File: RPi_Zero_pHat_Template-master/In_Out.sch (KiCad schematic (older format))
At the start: 34 parts, among them J3 DHT22 Conn, J4 HD38 Conn, J5 120VAC, J6 R_Si, J7 Ventilador, J8 Bomba Agua, J9 Tira LED, Q1 BT136-500, Q2 MMBT2222A, Q3 MMBT2222A, U4 LM35, U5 MOC3011M, U8 TLP3543

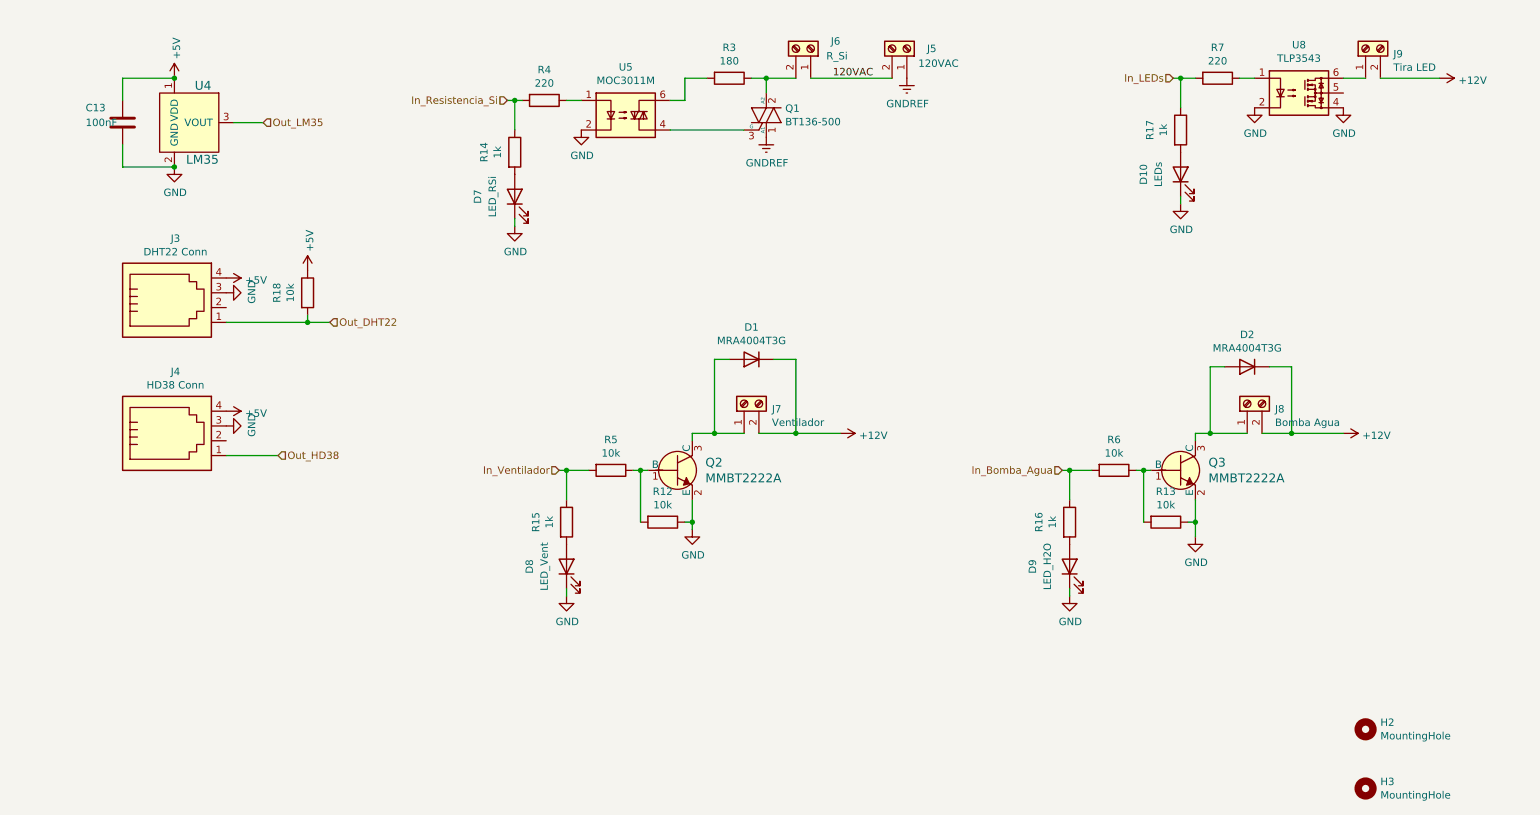
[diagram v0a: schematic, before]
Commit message: Archivos KiCad
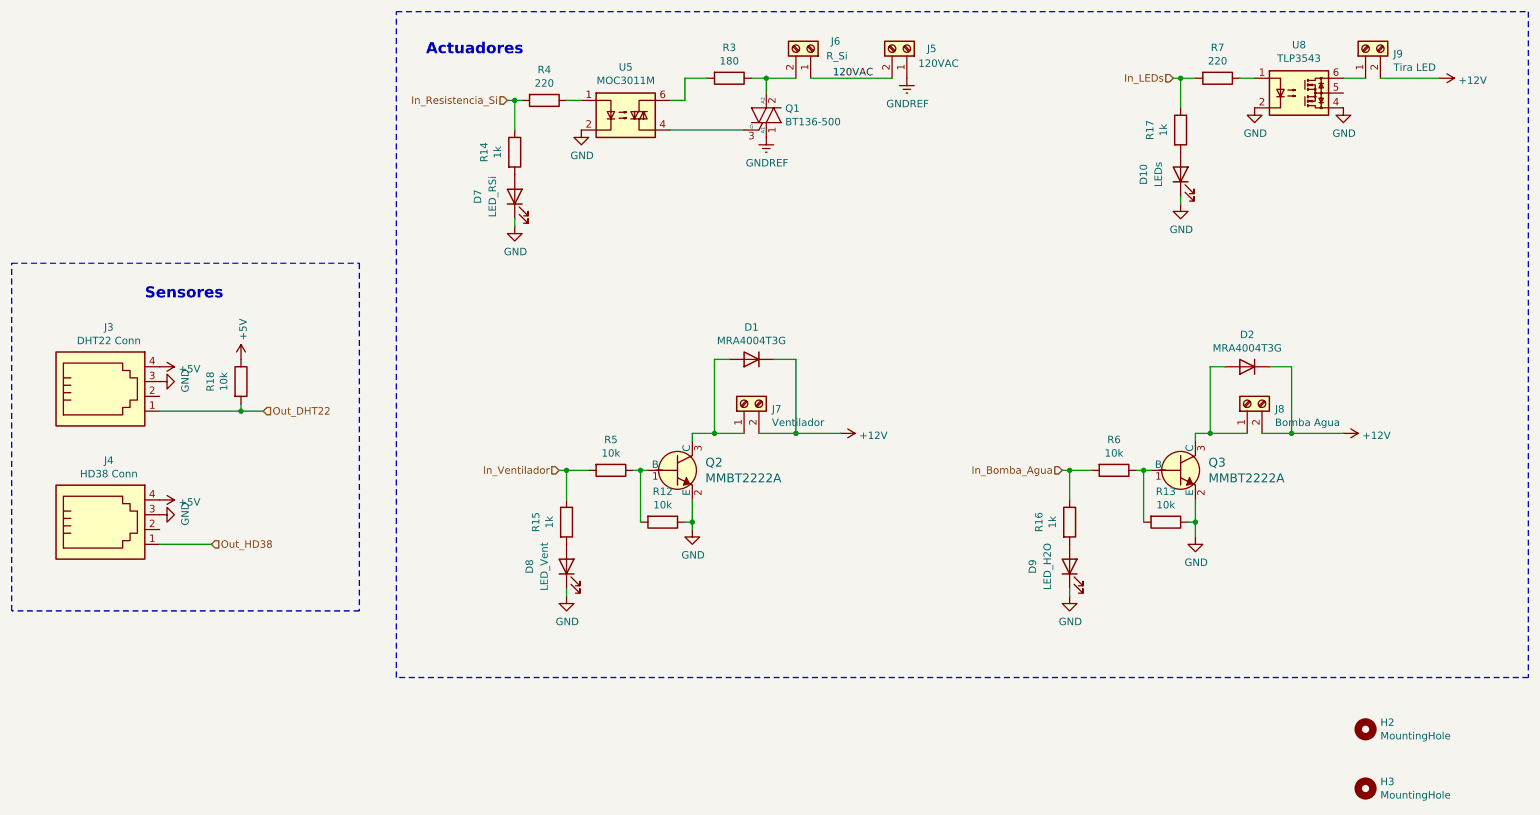
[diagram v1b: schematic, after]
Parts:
- removed C13: 100nF, Capacitor_SMD:C_0805_2012Metric, symbol Device:C
- removed U4: LM35, digikey-footprints:SOIC-8_W3.9mm, symbol dk_Temperature-Sensors-Analog-and-Digital-Output:LM35DT_NOPB
- J3, J4: footprint RJ9-Conn:520249-2 -> RJ9-Conn:RJ9-4P4C
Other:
- note added: "Actuadores"
- note added: "Sensores"
- moved on the sheet: J3, J4, R18
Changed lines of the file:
@@
 $EndDescr
-$Comp
-L dk_Temperature-Sensors-Analog-and-Digital-Output:LM35DT_NOPB U?
-U 1 1 608216FC
-P 1800 1500
-AR Path="/608216FC" Ref="U?"  Part="1"
-AR Path="/6081C49D/608216FC" Ref="U4"  Part="1"
-F 0 "U4" H 2050 1750 60  0000 R CNN
-F 1 "LM35" H 2100 1250 60  0000 R CNN
-F 2 "digikey-footprints:SOIC-8_W3.9mm" H 2000 1700 60  0001 L CNN
-F 3 "http://www.ti.com/general/docs/suppproductinfo.tsp?distId=10&gotoUrl=http%3A%2F%2Fwww.ti.com%2Flit%2Fgpn%2Flm35" H 2000 1800 60  0001 L CNN
-F 4 "LM35DT/NOPB-ND" H 2000 1900 60  0001 L CNN "Digi-Key_PN"
-F 5 "LM35DT/NOPB" H 2000 2000 60  0001 L CNN "MPN"
-F 6 "Sensors, Transducers" H 2000 2100 60  0001 L CNN "Category"
-F 7 "Temperature Sensors - Analog and Digital Output" H 2000 2200 60  0001 L CNN "Family"
-F 8 "http://www.ti.com/general/docs/suppproductinfo.tsp?distId=10&gotoUrl=http%3A%2F%2Fwww.ti.com%2Flit%2Fgpn%2Flm35" H 2000 2300 60  0001 L CNN "DK_Datasheet_Link"
-F 9 "/product-detail/en/texas-instruments/LM35DT-NOPB/LM35DT-NOPB-ND/362706" H 2000 2400 60  0001 L CNN "DK_Detail_Page"
-F 10 "SENSOR ANALOG 0C-100C TO220-3" H 2000 2500 60  0001 L CNN "Description"
-F 11 "Texas Instruments" H 2000 2600 60  0001 L CNN "Manufacturer"
-F 12 "Active" H 2000 2700 60  0001 L CNN "Status"
-	1    1800 1500
-	1    0    0    -1
-$EndComp
-$Comp
-L power:+5V #PWR?
-U 1 1 60821702
-P 1800 1200
-AR Path="/60821702" Ref="#PWR?"  Part="1"
-AR Path="/6081C49D/60821702" Ref="#PWR0130"  Part="1"
-F 0 "#PWR0130" H 1800 1050 50  0001 C CNN
-F 1 "+5V" V 1815 1328 50  0000 L CNN
-F 2 "" H 1800 1200 50  0001 C CNN
-F 3 "" H 1800 1200 50  0001 C CNN
-	1    1800 1200
-	1    0    0    -1
-$EndComp
-$Comp
-L power:GND #PWR?
-U 1 1 60821708
-P 1800 1800
-AR Path="/60821708" Ref="#PWR?"  Part="1"
-AR Path="/6081C49D/60821708" Ref="#PWR0131"  Part="1"
-F 0 "#PWR0131" H 1800 1550 50  0001 C CNN
-F 1 "GND" H 1805 1627 50  0000 C CNN
-F 2 "" H 1800 1800 50  0001 C CNN
-F 3 "" H 1800 1800 50  0001 C CNN
-	1    1800 1800
-	1    0    0    -1
-$EndComp
-Wire Wire Line
-	1450 1350 1450 1200
-Wire Wire Line
-	1450 1200 1800 1200
-Wire Wire Line
-	1450 1650 1450 1800
-Wire Wire Line
-	1450 1800 1800 1800
-Connection ~ 1800 1800
-$Comp
-L Device:C C?
-U 1 1 60821713
-P 1450 1500
-AR Path="/60821713" Ref="C?"  Part="1"
-AR Path="/6081C49D/60821713" Ref="C13"  Part="1"
-F 0 "C13" H 1200 1600 50  0000 L CNN
-F 1 "100nF" H 1200 1500 50  0000 L CNN
-F 2 "Capacitor_SMD:C_0805_2012Metric" H 1488 1350 50  0001 C CNN
-F 3 "~" H 1450 1500 50  0001 C CNN
-	1    1450 1500
-	1    0    0    -1
-$EndComp
-Connection ~ 1800 1200
-Wire Wire Line
-	2200 1500 2400 1500
-Text HLabel 2400 1500 2    50   Input ~ 0
-Out_LM35
 $Comp
 L Connector:4P4C J3
 U 1 1 607253E7
-P 1750 2750
-F 0 "J3" H 1807 3217 50  0000 C CNN
-F 1 "DHT22 Conn" H 1807 3126 50  0000 C CNN
-F 2 "RJ9-Conn:520249-2" V 1750 2800 50  0001 C CNN
-F 3 "~" V 1750 2800 50  0001 C CNN
-	1    1750 2750
+P 1300 3350
+F 0 "J3" H 1357 3817 50  0000 C CNN
+F 1 "DHT22 Conn" H 1357 3726 50  0000 C CNN
+F 2 "RJ9-Conn:RJ9-4P4C" V 1300 3400 50  0001 C CNN
+F 3 "~" V 1300 3400 50  0001 C CNN
+	1    1300 3350
 	1    0    0    -1
 $EndComp
@@
 L power:+5V #PWR0132
 U 1 1 60727756
-P 2150 2550
-F 0 "#PWR0132" H 2150 2400 50  0001 C CNN
-F 1 "+5V" V 2165 2678 50  0000 L CNN
-F 2 "" H 2150 2550 50  0001 C CNN
-F 3 "" H 2150 2550 50  0001 C CNN
-	1    2150 2550
+P 1700 3150
+F 0 "#PWR0132" H 1700 3000 50  0001 C CNN
+F 1 "+5V" V 1715 3278 50  0000 L CNN
+F 2 "" H 1700 3150 50  0001 C CNN
+F 3 "" H 1700 3150 50  0001 C CNN
+	1    1700 3150
 	0    1    1    0
 $EndComp
@@
 L power:GND #PWR?
 U 1 1 6072863A
-P 2150 2650
+P 1700 3250
 AR Path="/6072863A" Ref="#PWR?"  Part="1"
 AR Path="/6081C49D/6072863A" Ref="#PWR0133"  Part="1"
-F 0 "#PWR0133" H 2150 2400 50  0001 C CNN
-F 1 "GND" H 2155 2477 50  0000 C CNN
-F 2 "" H 2150 2650 50  0001 C CNN
-F 3 "" H 2150 2650 50  0001 C CNN
-	1    2150 2650
+F 0 "#PWR0133" H 1700 3000 50  0001 C CNN
+F 1 "GND" H 1705 3077 50  0000 C CNN
+F 2 "" H 1700 3250 50  0001 C CNN
+F 3 "" H 1700 3250 50  0001 C CNN
+	1    1700 3250
 	0    -1   -1   0
 $EndComp
-Text HLabel 2850 2850 2    50   Input ~ 0
+Text HLabel 2400 3450 2    50   Input ~ 0
 Out_DHT22
-Text HLabel 2500 3750 2    50   Input ~ 0
+Text HLabel 2050 4350 2    50   Input ~ 0
 Out_HD38
 Wire Wire Line
-	2150 3750 2500 3750
+	1700 4350 2050 4350
 $Comp
 L power:GND #PWR?
 U 1 1 60729FBF
-P 2150 3550
+P 1700 4150
 AR Path="/60729FBF" Ref="#PWR?"  Part="1"
 AR Path="/6081C49D/60729FBF" Ref="#PWR0134"  Part="1"
-F 0 "#PWR0134" H 2150 3300 50  0001 C CNN
-F 1 "GND" H 2155 3377 50  0000 C CNN
-F 2 "" H 2150 3550 50  0001 C CNN
-F 3 "" H 2150 3550 50  0001 C CNN
-	1    2150 3550
+F 0 "#PWR0134" H 1700 3900 50  0001 C CNN
+F 1 "GND" H 1705 3977 50  0000 C CNN
+F 2 "" H 1700 4150 50  0001 C CNN
+F 3 "" H 1700 4150 50  0001 C CNN
+	1    1700 4150
 	0    -1   -1   0
 $EndComp
@@
 L power:+5V #PWR0135
 U 1 1 60729C51
-P 2150 3450
-F 0 "#PWR0135" H 2150 3300 50  0001 C CNN
-F 1 "+5V" V 2165 3578 50  0000 L CNN
-F 2 "" H 2150 3450 50  0001 C CNN
-F 3 "" H 2150 3450 50  0001 C CNN
-	1    2150 3450
+P 1700 4050
+F 0 "#PWR0135" H 1700 3900 50  0001 C CNN
+F 1 "+5V" V 1715 4178 50  0000 L CNN
+F 2 "" H 1700 4050 50  0001 C CNN
+F 3 "" H 1700 4050 50  0001 C CNN
+	1    1700 4050
 	0    1    1    0
 $EndComp
@@
 L Connector:4P4C J4
 U 1 1 60729213
-P 1750 3650
-F 0 "J4" H 1807 4117 50  0000 C CNN
-F 1 "HD38 Conn" H 1807 4026 50  0000 C CNN
-F 2 "RJ9-Conn:520249-2" V 1750 3700 50  0001 C CNN
-F 3 "~" V 1750 3700 50  0001 C CNN
-	1    1750 3650
+P 1300 4250
+F 0 "J4" H 1357 4717 50  0000 C CNN
+F 1 "HD38 Conn" H 1357 4626 50  0000 C CNN
+F 2 "RJ9-Conn:RJ9-4P4C" V 1300 4300 50  0001 C CNN
+F 3 "~" V 1300 4300 50  0001 C CNN
+	1    1300 4250
 	1    0    0    -1
 $EndComp
@@
 L Device:R R18
 U 1 1 608294FE
-P 2700 2650
+P 2250 3250
 AR Path="/6081C49D/608294FE" Ref="R18"  Part="1"
 AR Path="/607B7D6E/608294FE" Ref="R?"  Part="1"
 AR Path="/60760232/608294FE" Ref="R?"  Part="1"
 AR Path="/60805E76/608294FE" Ref="R?"  Part="1"
-F 0 "R18" V 2493 2650 50  0000 C CNN
-F 1 "10k" V 2584 2650 50  0000 C CNN
-F 2 "Resistor_SMD:R_0805_2012Metric" V 2630 2650 50  0001 C CNN
-F 3 "~" H 2700 2650 50  0001 C CNN
-	1    2700 2650
+F 0 "R18" V 2043 3250 50  0000 C CNN
+F 1 "10k" V 2134 3250 50  0000 C CNN
+F 2 "Resistor_SMD:R_0805_2012Metric" V 2180 3250 50  0001 C CNN
+F 3 "~" H 2250 3250 50  0001 C CNN
+	1    2250 3250
 	1    0    0    -1
 $EndComp
@@
 L power:+5V #PWR0154
 U 1 1 608298A0
-P 2700 2500
-F 0 "#PWR0154" H 2700 2350 50  0001 C CNN
-F 1 "+5V" V 2715 2628 50  0000 L CNN
-F 2 "" H 2700 2500 50  0001 C CNN
-F 3 "" H 2700 2500 50  0001 C CNN
-	1    2700 2500
-	1    0    0    -1
-$EndComp
-Wire Wire Line
-	2700 2800 2700 2850
-Wire Wire Line
-	2150 2850 2700 2850
-Wire Wire Line
-	2850 2850 2700 2850
-Connection ~ 2700 2850
+P 2250 3100
+F 0 "#PWR0154" H 2250 2950 50  0001 C CNN
+F 1 "+5V" V 2265 3228 50  0000 L CNN
+F 2 "" H 2250 3100 50  0001 C CNN
+F 3 "" H 2250 3100 50  0001 C CNN
+	1    2250 3100
+	1    0    0    -1
+$EndComp
+Wire Wire Line
+	2250 3400 2250 3450
+Wire Wire Line
+	1700 3450 2250 3450
+Wire Wire Line
+	2400 3450 2250 3450
+Connection ~ 2250 3450
 Wire Wire Line
 	5850 3100 6000 3100
@@
 	-1   0    0    1
 $EndComp
+Wire Notes Line
+	3050 2450 3050 4800
+Wire Notes Line
+	3050 4800 700  4800
+Wire Notes Line
+	700  4800 700  2450
+Wire Notes Line
+	700  2450 3050 2450
+Text Notes 1600 2700 0    75   ~ 15
+Sensores
+Wire Notes Line
+	10950 750  10950 5250
+Wire Notes Line
+	10950 5250 3300 5250
+Wire Notes Line
+	3300 5250 3300 750
+Wire Notes Line
+	3300 750  10950 750
+Text Notes 3500 1050 0    75   ~ 15
+Actuadores
 $EndSCHEMATC
